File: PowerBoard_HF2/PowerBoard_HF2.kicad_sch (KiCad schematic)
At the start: 24 parts, among them J1 Power Supply

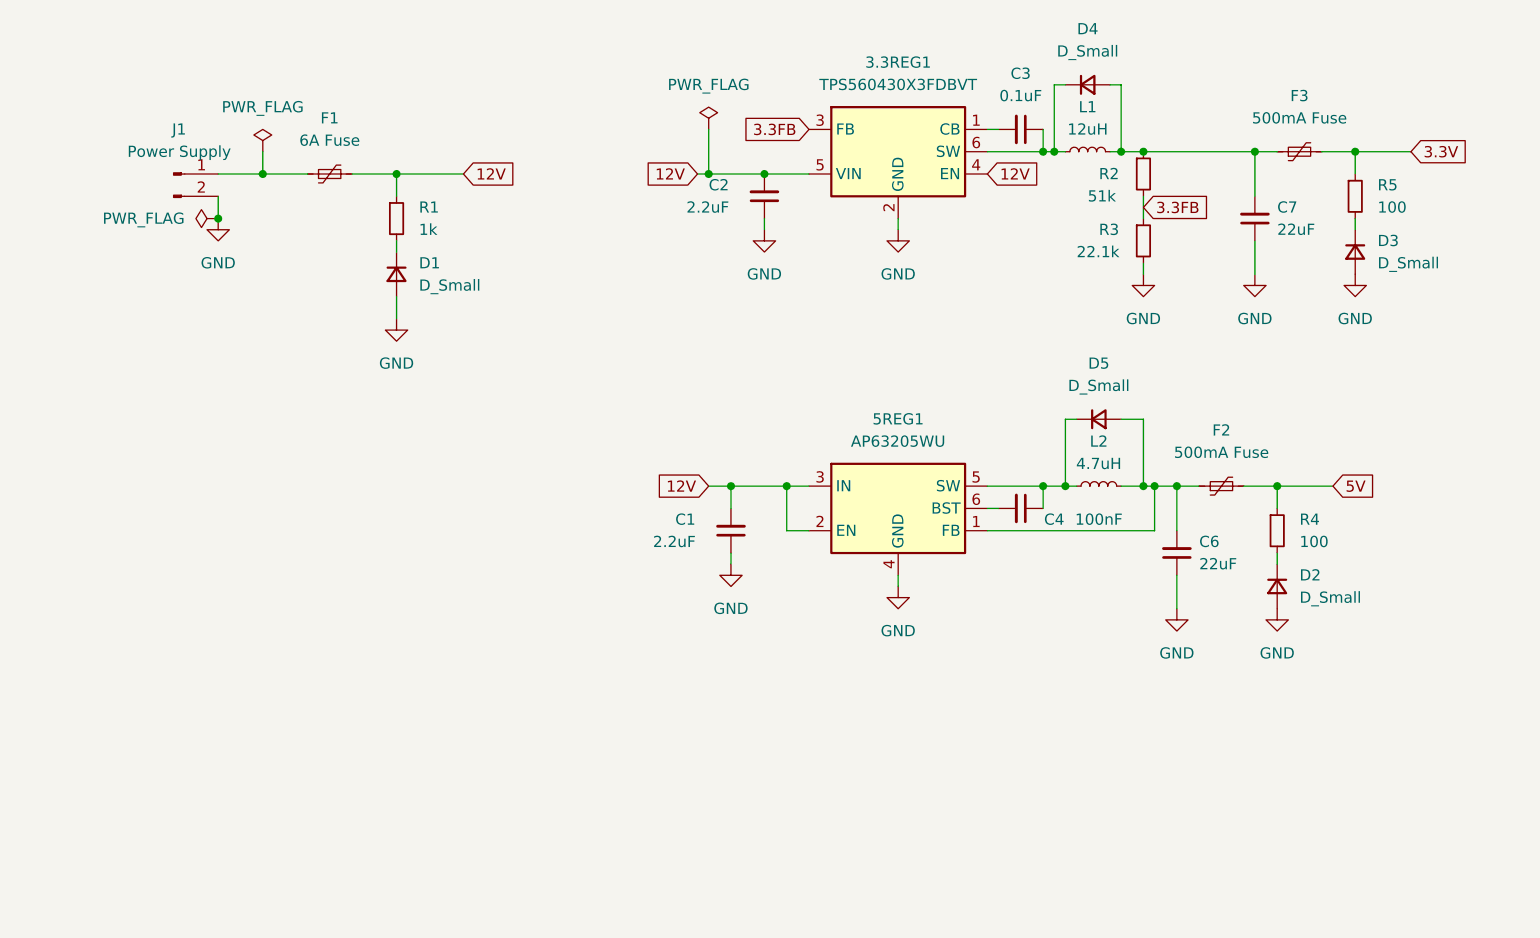
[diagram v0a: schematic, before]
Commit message: board updates
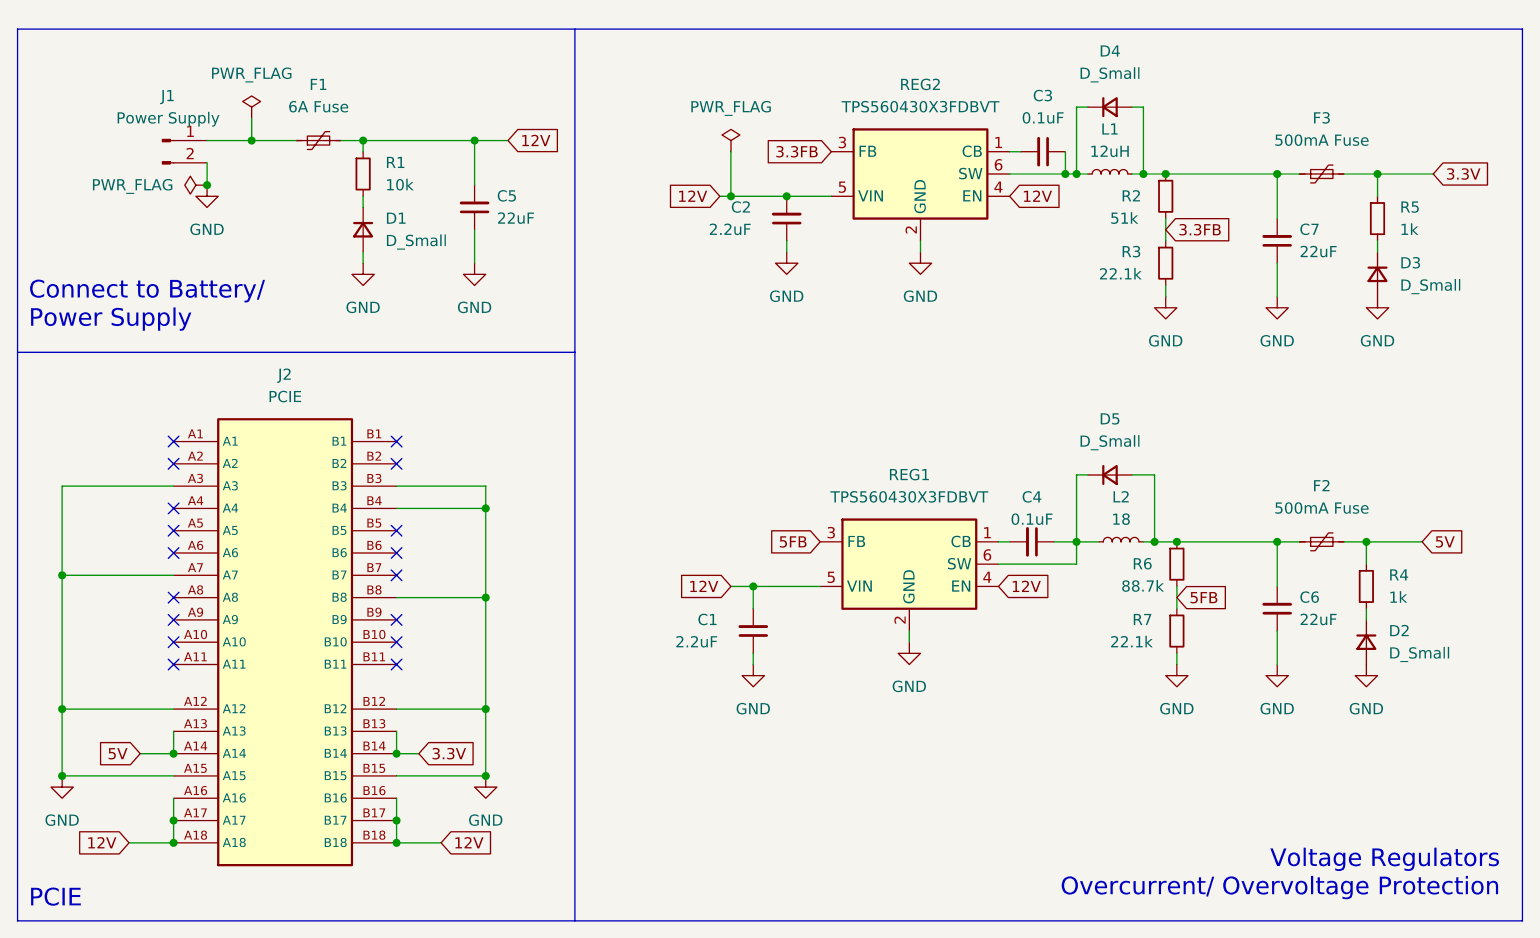
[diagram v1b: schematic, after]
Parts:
- removed 5REG1: AP63205WU, Package_TO_SOT_SMD:TSOT-23-6, symbol Regulator_Switching:AP63205WU
- added C5: 22uF, symbol Device:C_Small
- added J2: PCIE, symbol PCIE:PCIE-LP-01-01-F-DV-A-TR_(card_edge)
- added R6: 88.7k, symbol Device:R_Small
- added R7: 22.1k, symbol Device:R_Small
- added REG1: TPS560430X3FDBVT, Package_TO_SOT_SMD:SOT-23-6, symbol Regulator_Switching:TPS560430X3FDBVT
- C4: value 100nF -> 0.1uF
- L2: value 4.7uH -> 18
- R1: value 1k -> 10k
- R4, R5: value 100 -> 1k
- renumbered 3.3REG1 to REG2
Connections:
- net 12V: now also C5.2, J2.A16, J2.A17, J2.A18, J2.B16, J2.B17, J2.B18, REG1.4 (EN), REG1.5 (VIN)
- net 3.3V: now also J2.B13, J2.B14
- net 5V: now also J2.A13, J2.A14
- net GND: now also C5.1, J2.A12, J2.A15, J2.A3, J2.A7, J2.B12, J2.B15, J2.B3, J2.B4, J2.B8, R7.2, REG1.2 (GND)
- net at C6.2, D5.2 (A), F2.1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: now also R6.1
- net at C4.1, D5.1 (K), L2.1: now also REG1.6 (SW)
- net at C4.2: now also REG1.1 (CB)
- new net 5FB: R6.2, R7.1, REG1.3 (FB)
- no-connect marks 0 -> 17
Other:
- note added: "Connect to Battery/ Power Supply"
- note added: "PCIE"
- note added: "Voltage Regulators Overcurrent/ Overvoltage Protection"
- moved on the sheet: C1, C2, C3, C4, C6, C7, D1, D2, D3, D4, D5, F1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
